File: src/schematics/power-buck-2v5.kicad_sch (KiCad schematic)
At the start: 12 parts, among them U16 INA219xxDCN, U3 TPS562202DRLR

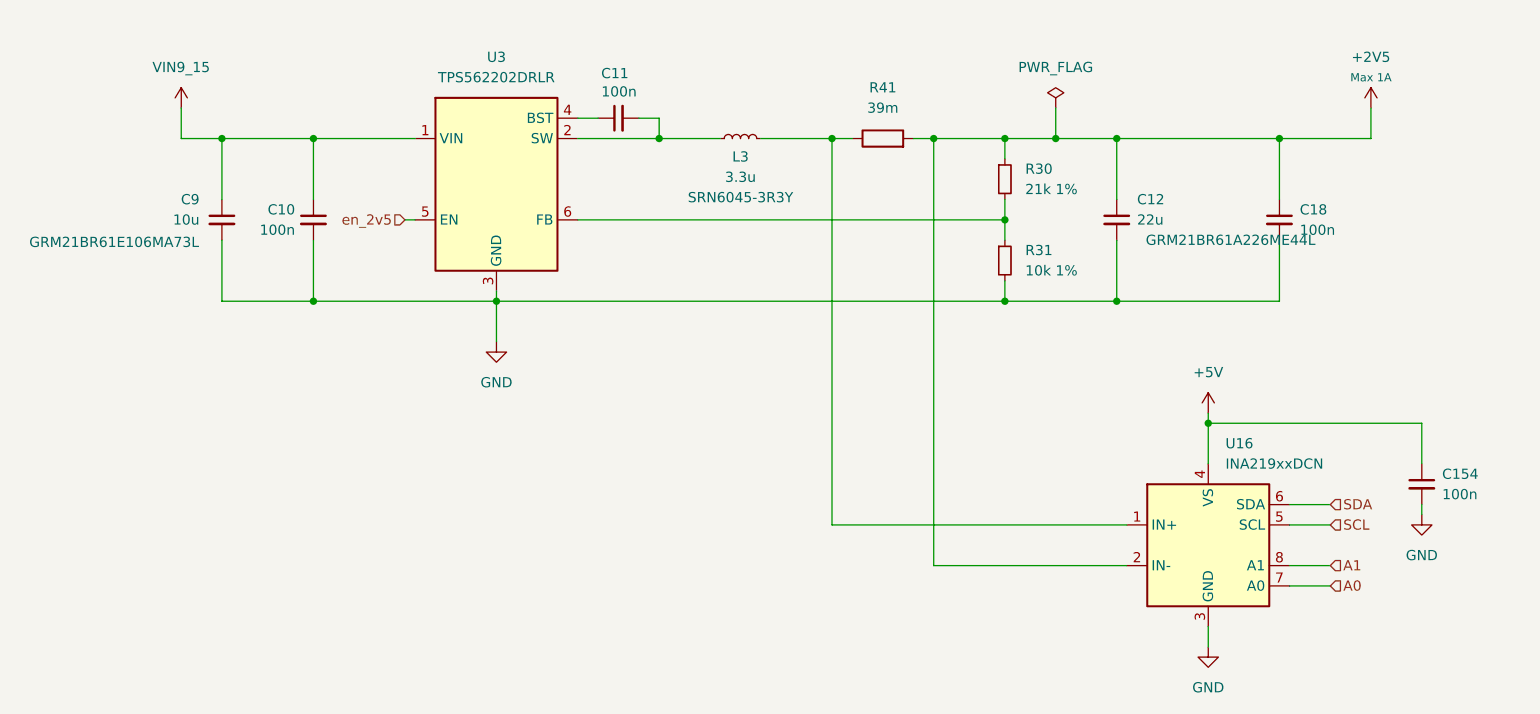
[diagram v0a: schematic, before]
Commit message: Add bom components
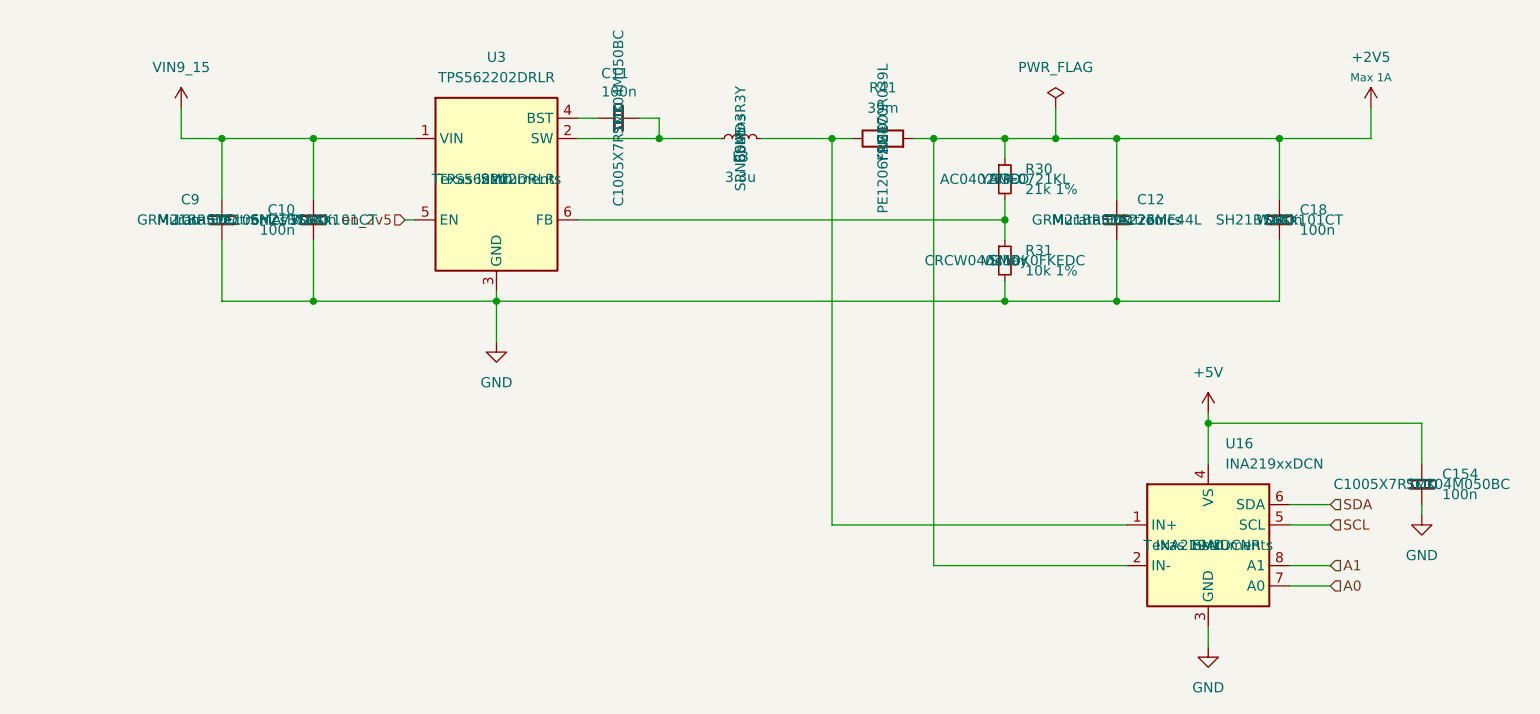
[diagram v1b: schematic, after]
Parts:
- C10, C18: MPN (none) -> SH21B104K101CT; Manufacturer (none) -> Walsin; Mouting Technology (none) -> SMD
- C11, C154: MPN (none) -> C1005X7R1C104M050BC; Manufacturer (none) -> TDK; Mouting Technology (none) -> SMD
- C12: MPN (none) -> GRM21BR61A226ME44L; Manufacturer (none) -> Murata Electronics; Mouting Technology (none) -> SMD; Part GRM21BR61A226ME44L -> (none)
- C9: MPN (none) -> GRM21BR61E106MA73L; Manufacturer (none) -> Murata Electronics; Mouting Technology (none) -> SMD; Part GRM21BR61E106MA73L -> (none)
- L3: MPN (none) -> SRN6045-3R3Y; Manufacturer (none) -> Bourns; Mouting Technology (none) -> SMD; Part SRN6045-3R3Y -> (none)
- R30: MPN (none) -> AC0402FR-0721KL; Manufacturer (none) -> YAGEO; Mouting Technology (none) -> SMD
- R31: MPN (none) -> CRCW040210K0FKEDC; Manufacturer (none) -> Vishay; Mouting Technology (none) -> SMD
- R41: MPN (none) -> PE1206FRE470R039L; Manufacturer (none) -> YAGEO; Mouting Technology (none) -> SMD
- U16: MPN (none) -> INA219AIDCNR; Manufacturer (none) -> Texas Instruments; Mouting Technology (none) -> SMD
- U3: MPN (none) -> TPS562202DRLR; Manufacturer (none) -> Texas Instruments; Mouting Technology (none) -> SMD
